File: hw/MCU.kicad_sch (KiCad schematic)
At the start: 53 parts, among them J1 BAT_9V, J2 SWD, J3 USB_C_Receptacle_USB2.0, Q1 2N7002, SW1 SW_Push, U1 AMS1117-5.0, U1 XC6220B331MR, U2 W25Q128JVSS, U3 RP2040, Y1 12MHz

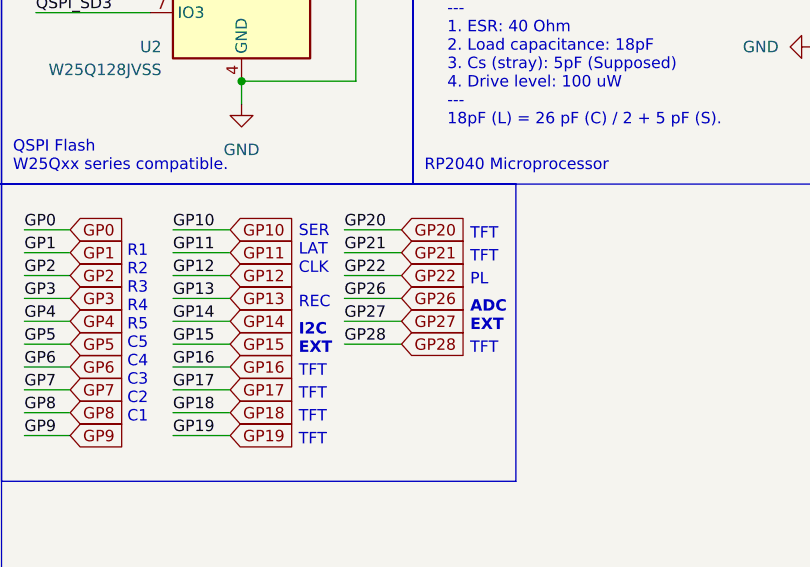
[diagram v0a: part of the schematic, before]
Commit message: Schematic updated.
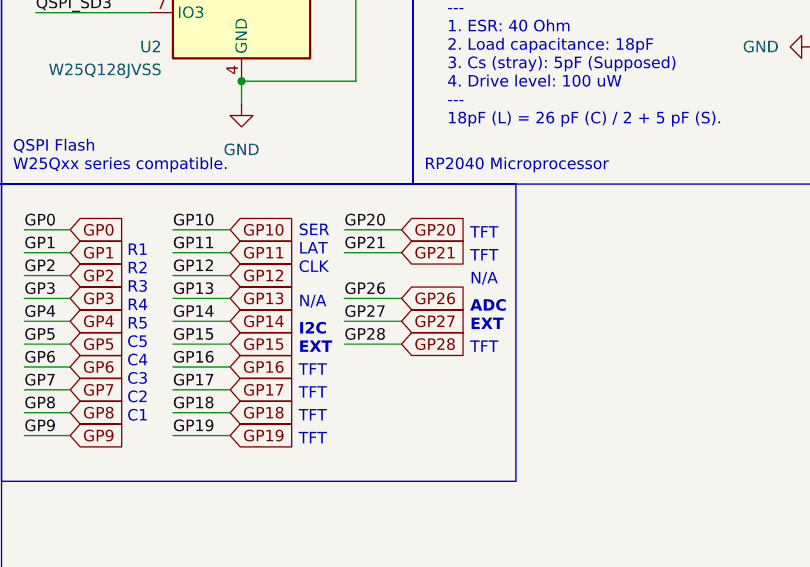
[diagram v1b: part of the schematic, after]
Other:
- note added: "N/A"
- note removed: "PL"
- note removed: "REC"
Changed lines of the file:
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@@
-    (stroke (width 0) (type default))
-  )
-  (wire (pts (xy 152.4 151.13) (xy 158.75 151.13))
     (stroke (width 0) (type default))
   )
@@
     (effects (font (size 1.27 1.27)) (justify left bottom))
   )
-  (text "PL" (at 166.37 152.4 0)
-    (effects (font (size 1.27 1.27)) (justify left bottom))
-  )
-  (text "REC" (at 147.32 154.94 0)
+  (text "N/A" (at 166.37 152.4 0)
+    (effects (font (size 1.27 1.27)) (justify left bottom))
+  )
+  (text "N/A" (at 147.32 154.94 0)
     (effects (font (size 1.27 1.27)) (justify left bottom))
   )
@@
   (label "VSYS" (at 101.6 93.98 270) (fields_autoplaced)
     (effects (font (size 1.27 1.27)) (justify right bottom))
-  )
-  (label "GP22" (at 152.4 151.13 0) (fields_autoplaced)
-    (effects (font (size 1.27 1.27)) (justify left bottom))
   )
   (label "QSPI_SS" (at 118.11 109.22 0) (fields_autoplaced)
@@
       (effects (font (size 1.27 1.27)) (justify left) hide)
     )
-  )
-  (global_label "GP22" (shape input) (at 158.75 151.13 0) (fields_autoplaced)
-    (effects (font (size 1.27 1.27)) (justify left))
-    (property "Intersheetrefs" "${INTERSHEET_REFS}" (at 166.6942 151.13 0)
-      (effects (font (size 1.27 1.27)) (justify left) hide)
-    )
